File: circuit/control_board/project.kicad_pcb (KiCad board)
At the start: 4 copper layers, 95 x 50 mm, 121 parts, among them J1 ANT, J2 Conn_01x08, J3 Conn_01x04, M1 Debugger, SW1 SW_DIP_x02, U1 TAU1201, U10 CH440R, U11 RM3100_13156, U12 AT24C02, U13 MM32SPIN27PS, U14 π131M31, U2 XPT2046TS, U3 ADIS16470AMLZ, U4 HX9193, U5 B0505S-1WR3, U6 MM32F3277G9P, U7 HX9193, U8 HX9193, U9 MM32F3277G9P, Y1 8MHz, Y2 8MHz, Y3 8MHz

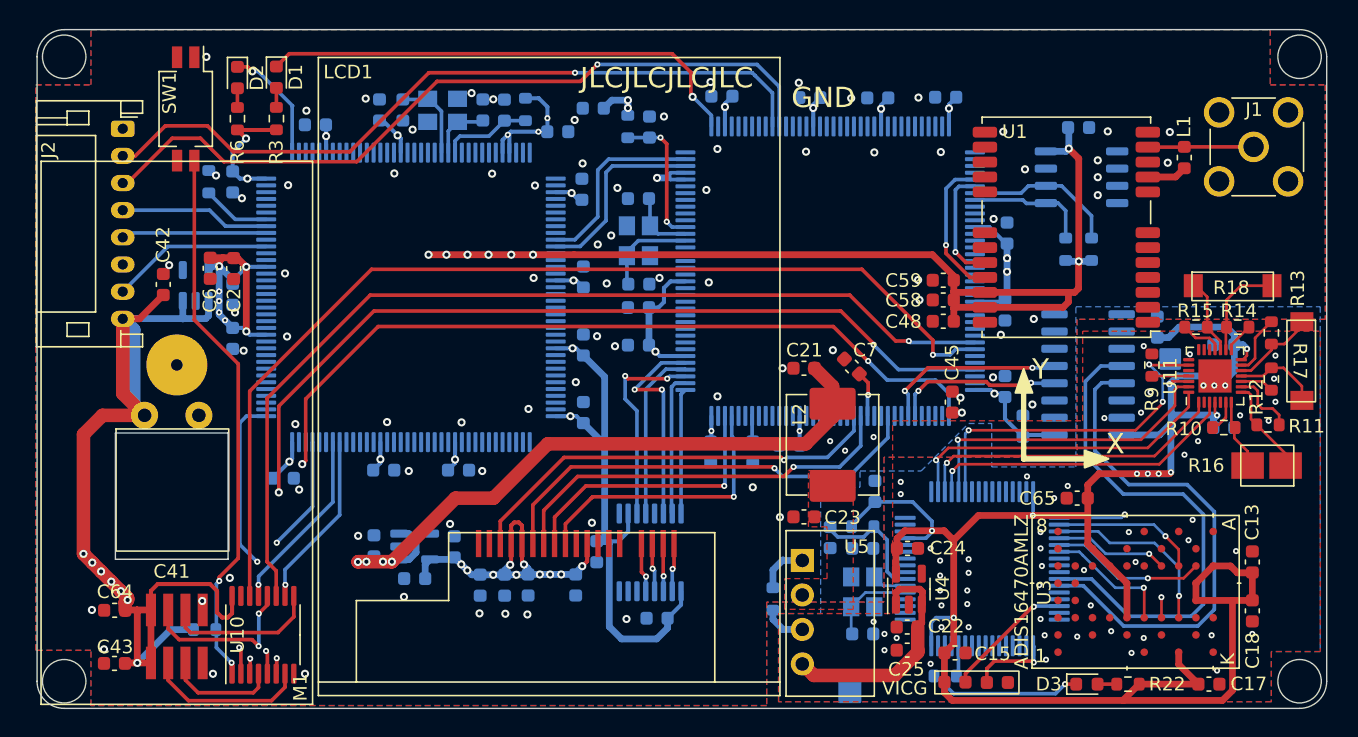
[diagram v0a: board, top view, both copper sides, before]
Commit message: Update the ControlBoard's PCB and export the interactive BOM.
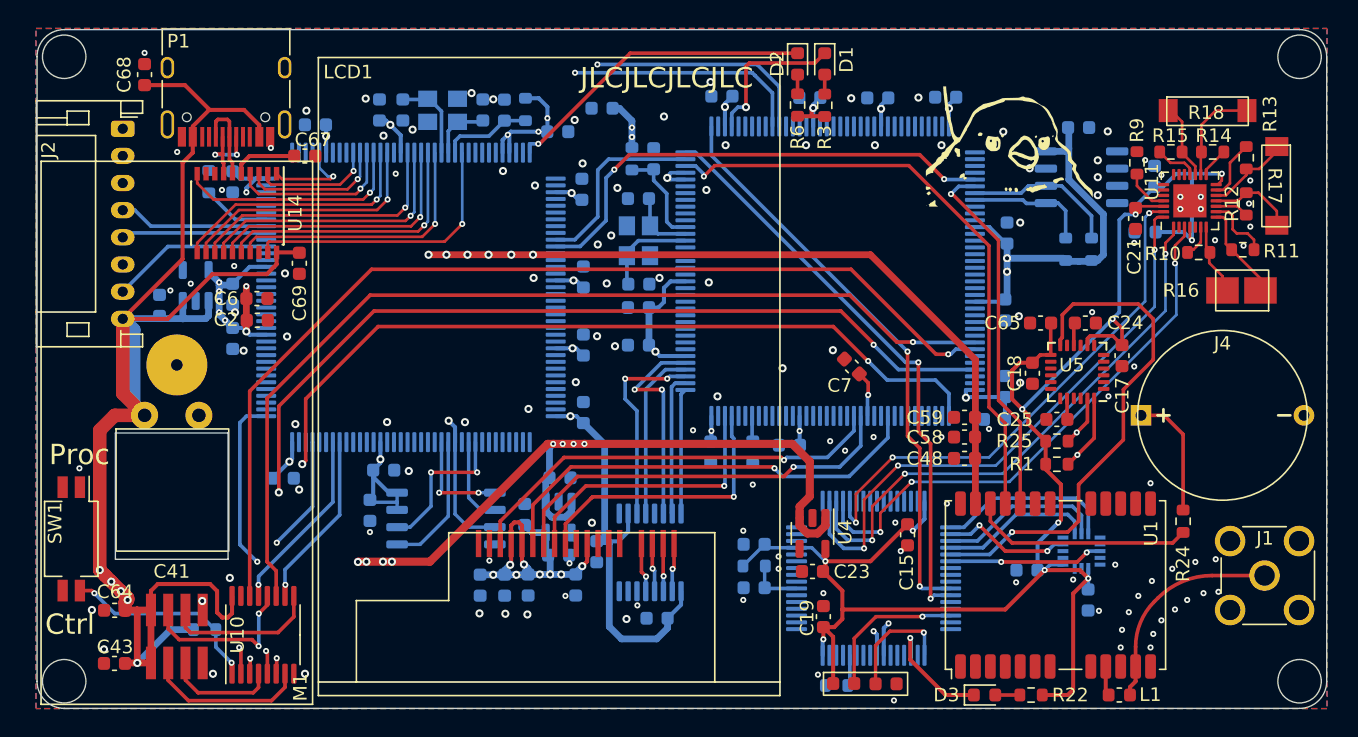
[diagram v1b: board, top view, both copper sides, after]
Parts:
- removed L2: 6.8uH, ControlBoard:L_Abracon_ASPI-0630LR
- removed Y3: 8MHz, ControlBoard:Crystal_SMD_3225-4Pin_3.2x2.5mm
- added G***: LOGO, LOGO, F.Cu at (175.5, 81.2)
- added J4: BAT_CR1220, ControlBoard:BAT_CR1220, F.Cu at (185.2, 101.0)
- added P1: USB_C_Plug_USB2.0, ControlBoard:USB_C_Receptacle_HRO_TYPE-C-31-M-12, F.Cu at (117.8, 76.5)
- added R24: 1kR, ControlBoard:R_0603_1608Metric, F.Cu at (188.3, 108.8)
- added R25: 10kR, ControlBoard:R_0603_1608Metric, F.Cu at (179.0, 102.9)
- added U15: W25Q64, Package_SO:SOIC-8_5.23x5.23mm_P1.27mm, B.Cu at (134.0, 108.6)
- C13, C42, C45: moved to B.Cu
- C19, C67, R1: moved to F.Cu
- C21, C23: value 10uF -> 100nF
- C22: value 100nF -> 22uF; moved to B.Cu
- C24: value 22uF -> 100nF
- C25: value 10uF -> 2.2nF
- C68: value 18pF -> 10uF; moved to F.Cu
- C69: value 18pF -> 100nF; moved to F.Cu
- U14: value π131M31 -> CH372C; footprint ControlBoard:SOIC-16_3.9x9.9mm_P1.27mm -> Package_SO:SSOP-20_4.4x6.5mm_P0.65mm; moved to F.Cu
- U3: value ADIS16470AMLZ -> ADXL350BCEZ; footprint ControlBoard:ADIS16470AMLZ -> ControlBoard:LGA-16-3.35mm_3.53mm; moved to B.Cu
- U5: value B0505S-1WR3 -> MPU-6050; footprint ControlBoard:SIP-4_B0505S_1WR3 -> Sensor_Motion:InvenSense_QFN-24_4x4mm_P0.5mm
- moved U14 63.8 mm to (118.6, 86.1), turned to -90 degrees
- moved C68 63.4 mm to (111.8, 75.9), turned to 90 degrees
- moved C67 56.5 mm to (123.6, 81.9), turned to 0 degrees
- moved C69 49.7 mm to (123.2, 89.8), turned to -90 degrees
- moved D2 41.3 mm to (159.9, 75.1)
- moved R6 41.3 mm to (159.9, 78.2)
- moved R3 40.4 mm to (161.9, 78.2)
- moved D1 40.4 mm to (161.9, 75.1)
- moved L1 39.9 mm to (183.6, 121.6), turned to 0 degrees
- moved C22 34.0 mm to (185.5, 87.5)
- moved SW1 32.8 mm to (106.4, 110.1)
- moved C19 32.6 mm to (161.8, 115.9), turned to 90 degrees
- moved J1 31.6 mm to (194.3, 112.8)
- moved C13 29.3 mm to (186.2, 83.4)
- moved C21 26.8 mm to (184.8, 86.5), turned to -90 degrees
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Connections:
- C13 pad 2: GNDA -> GND
- C14 pad 2: GNDA -> GND
- C15 pad 2: GNDA -> GND
- C16 pad 2: GNDA -> GND
- C17 pad 2: GNDA -> GND
- C18 pad 2: GNDA -> GND
- C19 pad 2: GNDA -> GND
- C20 pad 2: GNDA -> GND
- C21 pad 1: +5V -> +3.3VADC
- C22 pad 1: +5VA -> +3.3VADC
- C22 pad 2: GNDA -> GND
- C23 pad 1: Net-(C23-Pad1) -> +3.3VADC
- C24 pad 1: +3.3VADC -> Net-(C24-Pad1)
- C24 pad 2: GNDA -> GND
- C25 pad 1: +5VA -> Net-(C25-Pad1)
- C25 pad 2: GNDA -> GND
- C65 pad 2: GNDA -> GND
- C66 pad 1: +3.3VP -> +3.3VA
- C67 pad 1: +3.3VA -> Net-(C67-Pad1)
- C68 pad 1: /Coprocessor/XTAL_OUT -> +5V
- C68 pad 2: GNDA -> GND
- C69 pad 1: /Coprocessor/XTAL_IN -> +5V
- C69 pad 2: GNDA -> GND
- C70 pad 2: GNDA -> GND
- J3 pad 4: GNDA -> GND
- R1 pad 1: GND -> +3.3VADC
- R1 pad 2: GNDA -> /Coprocessor/IIC_SDA
- R19 pad 1: +3.3VP -> +3.3VA
- R20 pad 1: +3.3VP -> +3.3VA
- R21 pad 1: GNDA -> GND
- R3 pad 1: +3.3VP -> +3.3VA
- R6 pad 1: +3.3VP -> +3.3VA
- R9 pad 2: GNDA -> GND
- U1 pad 22: +3.3VP -> Net-(R24-Pad1)
- U11 pad 19: GNDA -> GND
- U11 pad 2: GNDA -> GND
- U11 pad 20: GNDA -> GND
- U11 pad 22: GNDA -> GND
- U11 pad 23: /Compass&Storage/Compass_DR -> unconnected-(U11-Pad23)
- U11 pad 29: GNDA -> GND
- U11 pad 5: GNDA -> GND
- U12 pad 8: +3.3VP -> +3.3VA
- U13 pad 12: GNDA -> GND
- U13 pad 22: /Compass&Storage/Compass_DR -> unconnected-(U13-Pad22)
- U13 pad 31: GNDA -> GND
- U13 pad 42: /Coprocessor/UART_TX -> /Coprocessor/UART1_TX
- U13 pad 43: /Coprocessor/UART_RX -> /Coprocessor/UART1_RX
- U13 pad 5: /Coprocessor/XTAL_IN -> unconnected-(U13-Pad5)
- U13 pad 51: unconnected-(U13-Pad51) -> /Coprocessor/LED1
- U13 pad 55: unconnected-(U13-Pad55) -> /Coprocessor/IIC_SDA
- U13 pad 56: unconnected-(U13-Pad56) -> /Coprocessor/IIC_CLK
- U13 pad 6: /Coprocessor/XTAL_OUT -> unconnected-(U13-Pad6)
- U13 pad 62: /Coprocessor/LED1 -> unconnected-(U13-Pad62)
- U13 pad 63: GNDA -> GND
- U14 pad 1: +3.3VA -> /Control_MCU/PE6
- U14 pad 10: unconnected-(U14-Pad10) -> /Control_MCU/PF3
- U14 pad 11: unconnected-(U14-Pad11) -> /Control_MCU/PF4
- U14 pad 12: /Coprocessor/UART_TX -> /Control_MCU/PF5
- U14 pad 13: /Coprocessor/UART_RX -> /Control_MCU/PF6
- U14 pad 14: unconnected-(U14-Pad14) -> /Control_MCU/PF7
- U14 pad 15: GNDA -> /Control_MCU/PF8
- U14 pad 16: +3.3VADC -> /Control_MCU/PF9
- U14 pad 2: GND -> /Control_MCU/PF0
- U14 pad 3: unconnected-(U14-Pad3) -> /Control_MCU/PF1
- U14 pad 4: /Coprocessor/UART1_RX -> /Control_MCU/PF2
- U14 pad 5: /Coprocessor/UART1_TX -> Net-(C67-Pad1)
- U14 pad 6: unconnected-(U14-Pad6) -> Net-(P1-PadA6)
- U14 pad 7: unconnected-(U14-Pad7) -> Net-(P1-PadA7)
- U14 pad 9: GNDA -> unconnected-(U14-Pad9)
- U4 pad 1: +5VA -> +5V
- U4 pad 2: GNDA -> GND
- U4 pad 3: +5VA -> +5V
- U5 pad 2: Net-(C23-Pad1) -> (no net)
- U5 pad 3: GNDA -> (no net)
- U5 pad 4: +5VA -> (no net)
- U6 pad 114: /Coprocessor/UART1_RX -> unconnected-(U6-Pad114)
- U6 pad 115: /Coprocessor/UART1_TX -> unconnected-(U6-Pad115)
- U6 pad 34: /Control_MCU/UART6_RX -> /LCD&GPS/GPS_RX
- U6 pad 36: unconnected-(U6-Pad36) -> /Coprocessor/UART1_RX
- U6 pad 37: /Process_MCU/LED1 -> /Coprocessor/UART1_TX
- U6 pad 40: unconnected-(U6-Pad40) -> /Process_MCU/LED1
- U6 pad 77: /LCD&GPS/GPS_RX -> /Control_MCU/UART6_RX
- U9 pad 1: /Control_MCU/LED1 -> unconnected-(U9-Pad1)
- U9 pad 10: unconnected-(U9-Pad10) -> /Control_MCU/PF0
- U9 pad 11: unconnected-(U9-Pad11) -> /Control_MCU/PF1
- U9 pad 12: unconnected-(U9-Pad12) -> /Control_MCU/PF2
- U9 pad 13: unconnected-(U9-Pad13) -> /Control_MCU/PF3
- U9 pad 14: unconnected-(U9-Pad14) -> /Control_MCU/PF4
- U9 pad 15: unconnected-(U9-Pad15) -> /Control_MCU/PF5
- U9 pad 18: unconnected-(U9-Pad18) -> /Control_MCU/PF6
- U9 pad 19: unconnected-(U9-Pad19) -> /Control_MCU/PF7
- U9 pad 20: unconnected-(U9-Pad20) -> /Control_MCU/PF8
- U9 pad 21: unconnected-(U9-Pad21) -> /Control_MCU/PF9
- U9 pad 22: unconnected-(U9-Pad22) -> /Control_MCU/PF10
- U9 pad 26: unconnected-(U9-Pad26) -> /Control_MCU/PC0
- U9 pad 36: unconnected-(U9-Pad36) -> /Control_MCU/LED1
- U9 pad 5: unconnected-(U9-Pad5) -> /Control_MCU/PE6
- U9 pad 81: unconnected-(U9-Pad81) -> /Control_MCU/SPI3_CLK
- U9 pad 82: unconnected-(U9-Pad82) -> /Control_MCU/SPI3_MISO
- U9 pad 85: unconnected-(U9-Pad85) -> /Control_MCU/SPI3_MOSI
- U9 pad 86: unconnected-(U9-Pad86) -> /Control_MCU/SPI3_NSS
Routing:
- net +5V: track 149.7 -> 195.4 mm, vias 11 -> 13
- net /Coprocessor/UART_TX: track 37.9 -> 0.00 mm
- net /Coprocessor/UART_RX: track 37.7 -> 0.00 mm
- net /LCD&GPS/GPS_RX: track 10.8 -> 45.0 mm
- net /Coprocessor/UART1_RX: track 12.5 -> 42.9 mm
- net /Coprocessor/UART1_TX: track 13.7 -> 42.6 mm
- net /Coprocessor/IIC_CLK: track 0.00 -> 28.2 mm, vias 0 -> 2
- net /Coprocessor/IIC_SDA: track 0.00 -> 27.9 mm, vias 0 -> 2
- net /Coprocessor/PC6: track 11.5 -> 37.4 mm
- net /Compass&Storage/Compass_DR: track 26.0 -> 0.00 mm, vias 3 -> 0
- net /Debugger/SEL: track 40.2 -> 14.9 mm
- net +3.3VP: track 175.3 -> 150.3 mm, vias 29 -> 26
- net /Process_MCU/LED1: track 36.1 -> 11.4 mm
- net /Control_MCU/UART6_RX: track 14.1 -> 36.3 mm, vias 0 -> 2
- net /Control_MCU/PC0: track 0.00 -> 20.9 mm, vias 0 -> 1
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- removed copper zone on B.Cu, net GNDA
- removed copper zone on F.Cu, net GNDA
- removed copper zone on In1.Cu, net GNDA
- removed copper zone on In2.Cu, net GNDA
- removed copper zone on F.Cu, net Net-(C23-Pad1)
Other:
- board text added: "Ctrl"
- board text added: "GDUT 2022/04/06"
- board text added: "Proc"
- board text added: "Version 1.5.2"
- board text removed: "GDUT 2022/03/03"
- board text removed: "GND"
- board text removed: "VICG"
- board text removed: "Version 1.3.3"
- board text removed: "X"
- board text removed: "Y"
